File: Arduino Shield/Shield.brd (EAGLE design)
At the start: 117.2 x 100 mm, 33 parts, among them IC1 317T, IC2 317T

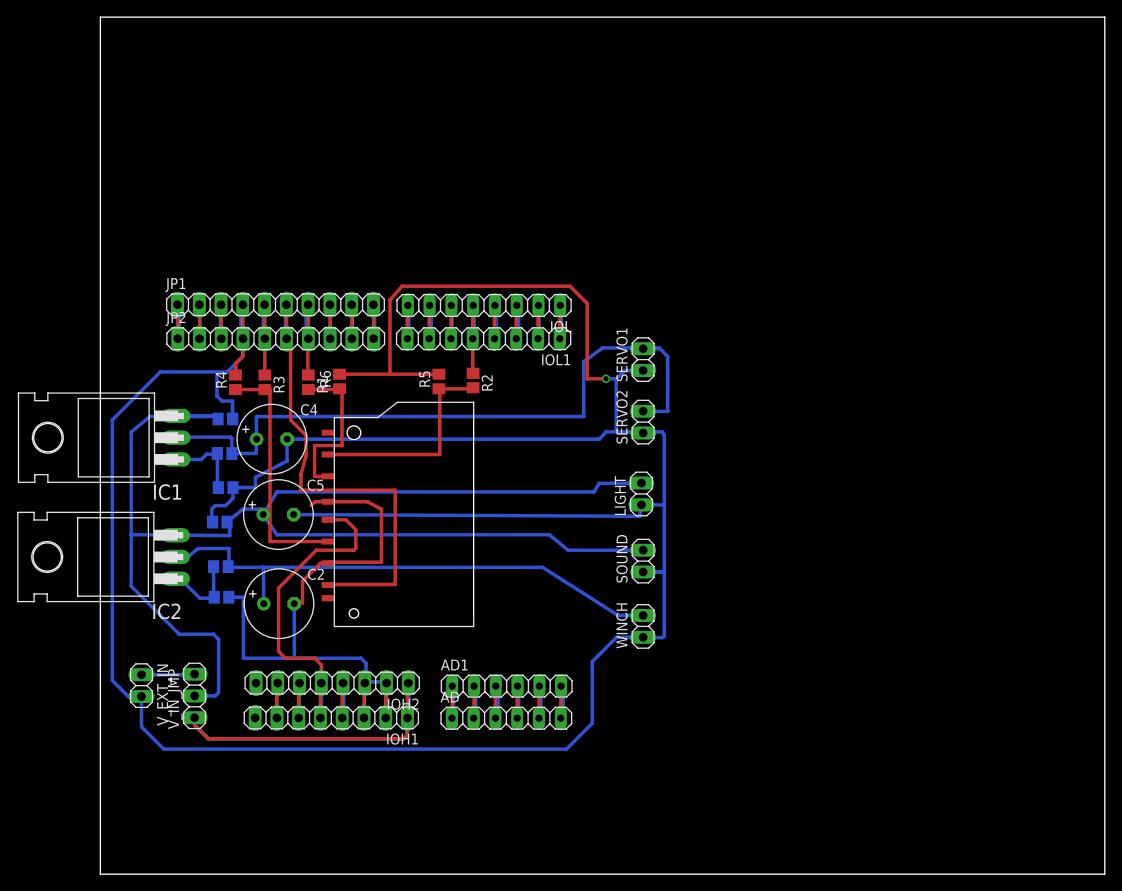
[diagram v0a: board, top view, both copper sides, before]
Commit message: Конечная разводка
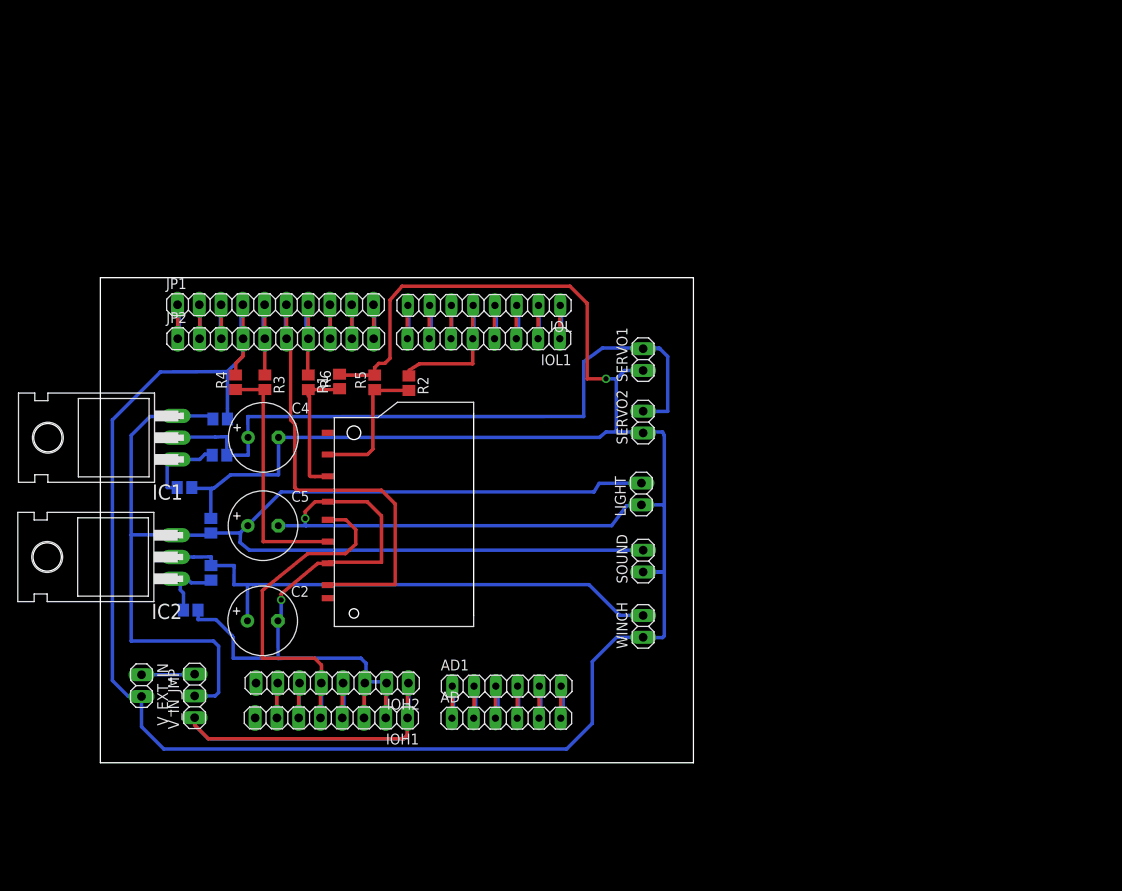
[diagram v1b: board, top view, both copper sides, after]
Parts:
- moved R2 7.51 mm to (78.8, 57.3)
- moved R5 7.50 mm to (74.8, 57.4)
- moved R8 4.80 mm to (52.6, 45.1)
- moved R10 3.90 mm to (53.3, 30.8)
- moved C2 2.76 mm to (61.7, 29.6)
- moved C5 2.22 mm to (61.8, 40.7)
- moved R9 1.36 mm to (55.7, 35.2), turned to 270 degrees
- moved C1 1.13 mm to (55.7, 40.7), turned to 90 degrees
- moved C4 1.02 mm to (61.8, 51.0)
- moved R7 0.63 mm to (56.7, 48.9)
- moved C3 0.60 mm to (56.8, 53.1)
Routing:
- net SD_CS: track 25.8 -> 16.5 mm
- net PIN4: track 8.09 -> 15.1 mm
- net GND: track 419.2 -> 423.2 mm, vias 1 -> 3
- net 3.3V: track 36.4 -> 39.9 mm
- net SD_DI: track 19.0 -> 16.4 mm
- net V_IN: track 167.4 -> 165.8 mm
- net PIN12: track 52.9 -> 51.9 mm
- net N$2: track 9.11 -> 8.27 mm
- net 6V: track 82.0 -> 82.7 mm
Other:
- board size 117.2 x 100 mm -> 69.2 x 56.6 mm
